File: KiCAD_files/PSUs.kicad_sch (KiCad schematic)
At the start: 12 parts

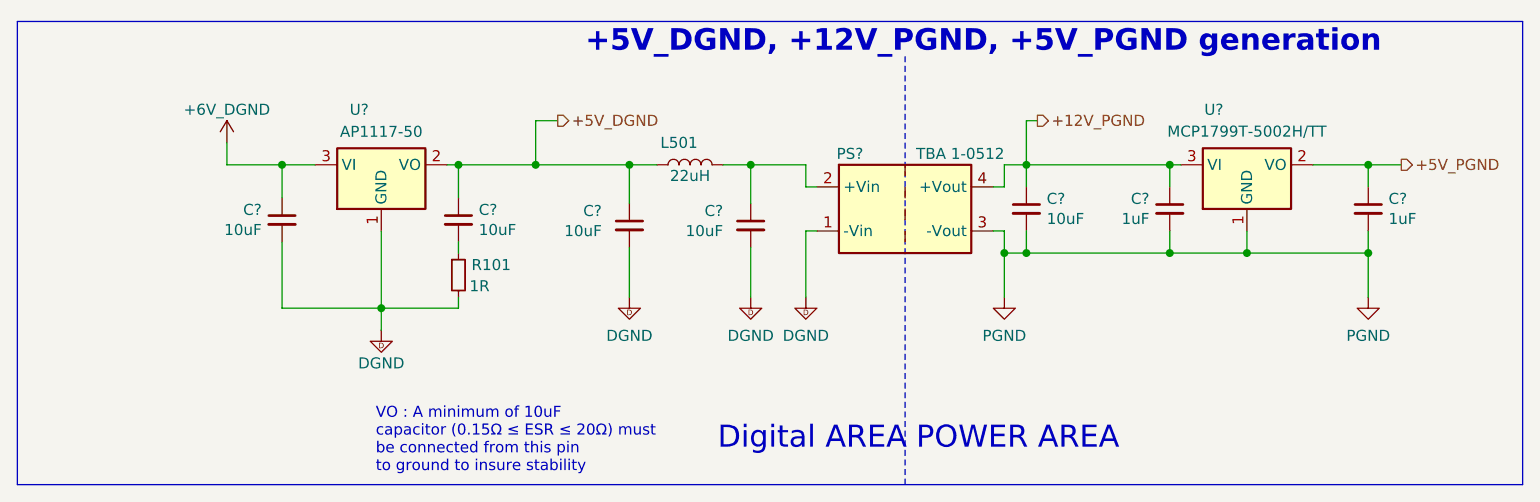
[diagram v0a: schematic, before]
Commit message: save before starting routing
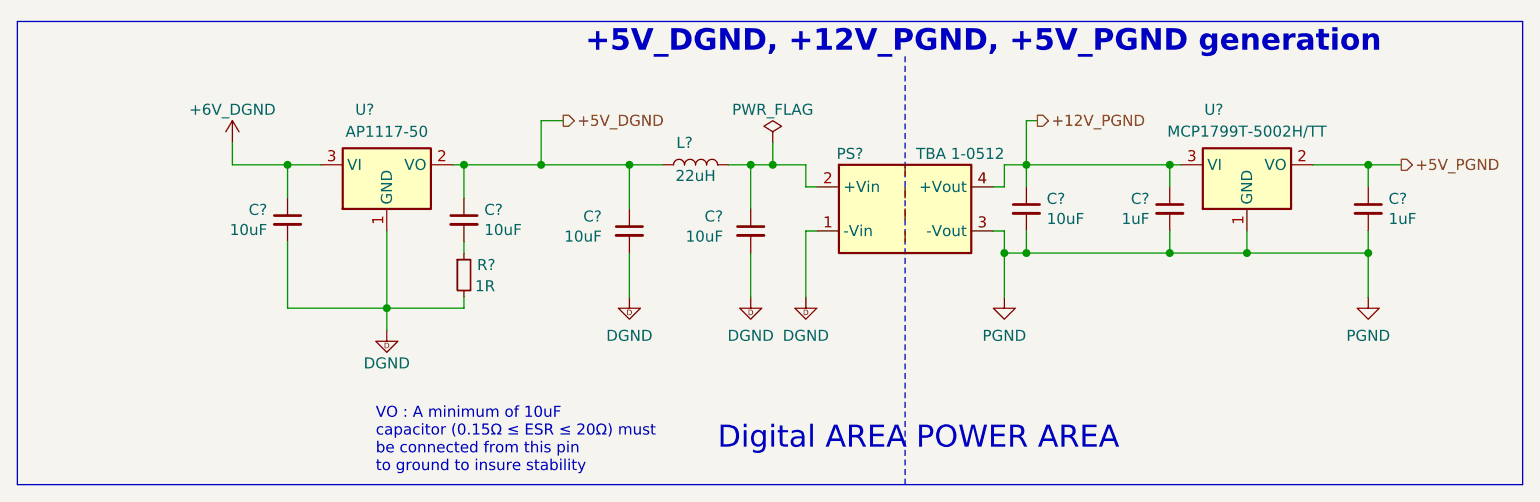
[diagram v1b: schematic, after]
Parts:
- L?: renamed from L501; footprint (none) -> Inductor_SMD:L_1210_3225Metric; manf# (none) -> CBC3225T220KR
- renumbered R101 to R?
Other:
- title: (none) -> OWNVERTER V0.1
- moved on the sheet: C?, L?, R?, U?

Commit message: dev
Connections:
- net GND renamed PGND
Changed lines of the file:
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@@
     )
   )
-  (symbol (lib_id "power:GND") (at 247.65 93.98 0) (mirror y) (unit 1)
+  (symbol (lib_id "Symbols:PGND") (at 247.65 93.98 0) (mirror y) (unit 1)
     (in_bom yes) (on_board yes) (dnp no) (fields_autoplaced)
     (property "Reference" "#PWR?" (at 247.65 100.33 0)
@@
     )
   )
-  (symbol (lib_id "power:GND") (at 205.74 93.98 0) (mirror y) (unit 1)
+  (symbol (lib_id "Symbols:PGND") (at 205.74 93.98 0) (mirror y) (unit 1)
     (in_bom yes) (on_board yes) (dnp no) (fields_autoplaced)
     (property "Reference" "#PWR?" (at 205.74 100.33 0)
